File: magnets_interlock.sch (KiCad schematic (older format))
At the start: 18 parts, among them U101 Si8640BD-B-IS

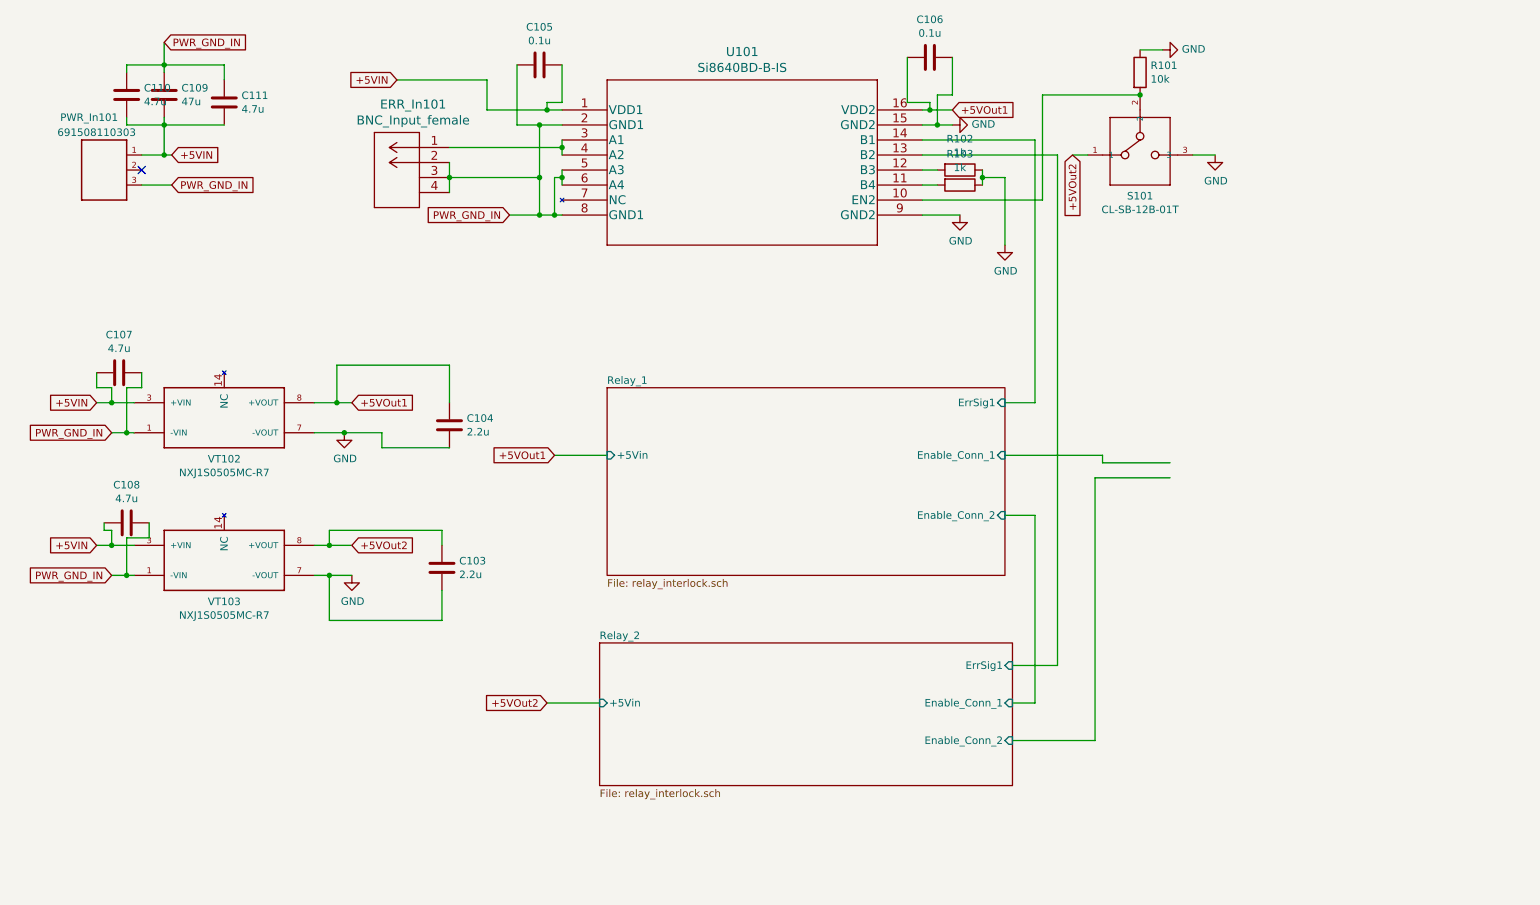
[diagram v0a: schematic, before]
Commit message: Draft 1 Almost There
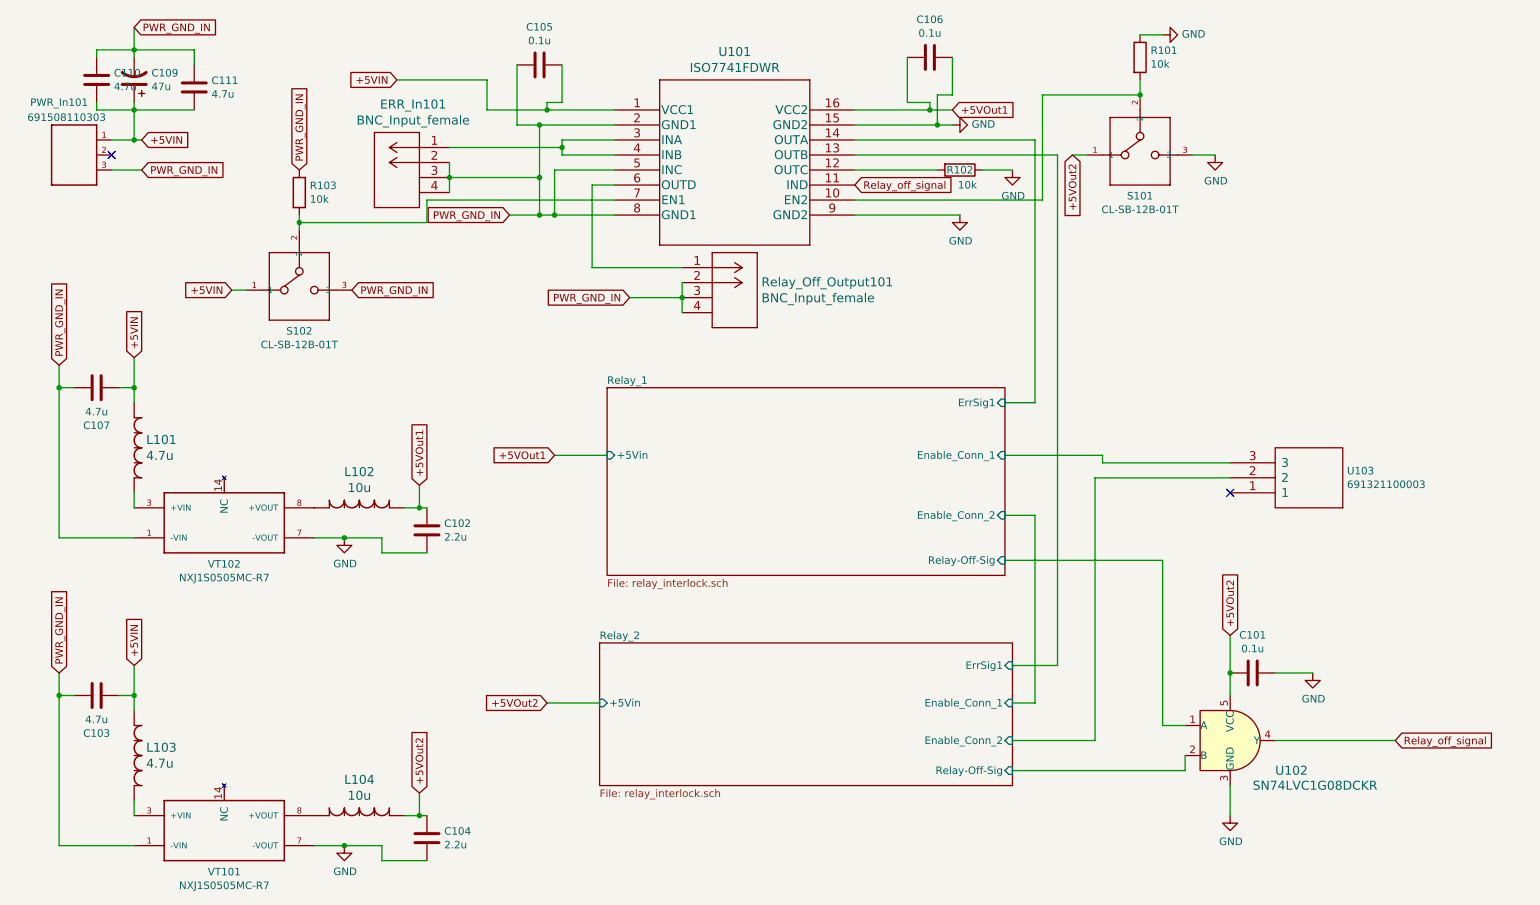
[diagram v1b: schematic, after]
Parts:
- removed C108: 4.7u, Capacitor_SMD:C_1206_3216Metric_Pad1.42x1.75mm_HandSolder, symbol Device:C
- removed C109: 47u, Capacitor_THT:CP_Radial_D8.0mm_P3.50mm, symbol Device:C
- removed U101: Si8640BD-B-IS, SI8640DBIS:Si8640BD-B-IS, symbol 2020-06-26_17-59-50:Si8640BD-B-IS
- removed VT103: NXJ1S0505MC-R7, NXJ1S050:VREG_NXJ1S0505MC-R7, symbol NXJ1S0505MC-R7:NXJ1S0505MC-R7
- added C101: 0.1u, Capacitor_SMD:C_1206_3216Metric_Pad1.42x1.75mm_HandSolder, symbol Device:C
- added C102: 2.2u, Capacitor_SMD:C_1206_3216Metric_Pad1.42x1.75mm_HandSolder, symbol Device:C
- added C109: 47u, Capacitor_THT:CP_Radial_D8.0mm_P3.50mm, symbol Device:CP1
- added L101, L103: 4.7u, VLCF4024T-4R7N1R4-2:VLCF4024T-4R7N1R4-2, symbol 2020-06-30_20-16-32:VLCF4024T-4R7N1R4-2
- added L102, L104: 10u, VLCF4024T-4R7N1R4-2:VLCF4024T-4R7N1R4-2, symbol 2020-06-30_19-50-11:VLCF4024T-100MR90-2
- added Relay_Off_Output101: BNC_Input_female, BNC_female:1-1337543-0, symbol magnets_interlock_library:BNC_Input_female
- added S102: CL-SB-12B-01T, CL-SB-12B-01T:CL-SB-12B, symbol CL-SB-12B-01T:CL-SB-12B-01T
- added U101: ISO7741FDWR, ISO7741FDWR:ISO7741FDWR, symbol 2020-06-30_17-30-58:ISO7741FDWR
- added U102: SN74LVC1G08DCKR, inverter:SN74LVC1G14DCKR, symbol dk_Logic-Gates-and-Inverters:SN74LVC1G08DCKR
- added U103: 691321100003, Magnet_PS_Interlock:691321100003, symbol enrique_3termscrew:691321100003
- added VT101: NXJ1S0505MC-R7, NXJ1S050:VREG_NXJ1S0505MC-R7, symbol NXJ1S0505MC-R7:NXJ1S0505MC-R7
- C103: value 2.2u -> 4.7u
- R102, R103: value 1k -> 10k
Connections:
- net +5VIN: now also C103.1, C109.1, L101.2, L103.2, S102.1, U101.1 (VCC1); no longer VT102.3 (+VIN)
- net +5VOut1: now also C102.1, L102.1, U101.16 (VCC2); no longer C104.1, VT102.8 (+VOUT)
- net +5VOut2: now also C104.1, C101.2, L104.1, U102.5 (VCC); no longer C103.1
- net GND: now also C101.1, C102.2, U101.15 (GND2), U101.9 (GND2), U102.3 (GND), VT101.7 (-VOUT); no longer C103.2, R103.1
- net PWR_GND_IN: now also C103.2, R103.1, C109.2, Relay_Off_Output101.2 (BNC_Shield), Relay_Off_Output101.3 (shield), Relay_Off_Output101.4 (shield), S102.3, U101.2 (GND1), U101.5 (INC), U101.8 (GND1), VT101.1 (-VIN)
- net Relay_1/Enable_Conn_1: now also U103.3
- net Relay_1/ErrSig1: now also U101.14 (OUTA)
- net Relay_2/Enable_Conn_2: now also U103.2
- net Relay_2/ErrSig1: now also U101.13 (OUTB)
- net at R101.2, S101.2: now also U101.10 (EN2)
- net at R103.2: now also S102.2, U101.7 (EN1)
- net at R102.2: now also U101.12 (OUTC)
- net at ERR_In101.1 (Center_Pin): now also U101.3 (INA), U101.4 (INB)
- new net: L101.1, VT102.3 (+VIN)
- new net: L102.2, VT102.8 (+VOUT)
- new net: L104.2, VT101.8 (+VOUT)
- new net: L103.1, VT101.3 (+VIN)
- new net: Relay_Off_Output101.1 (Center_Pin), U101.6 (OUTD)
- new net Relay_1/Relay-Off-Sig: U102.1 (A)
- new net Relay_2/Relay-Off-Sig: U102.2 (B)
- new net Relay_off_signal: U101.11 (IND), U102.4 (Y)
- no-connect marks 1 -> 2
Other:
- moved on the sheet: C107, C110, C111, PWR_In101, R101, VT102

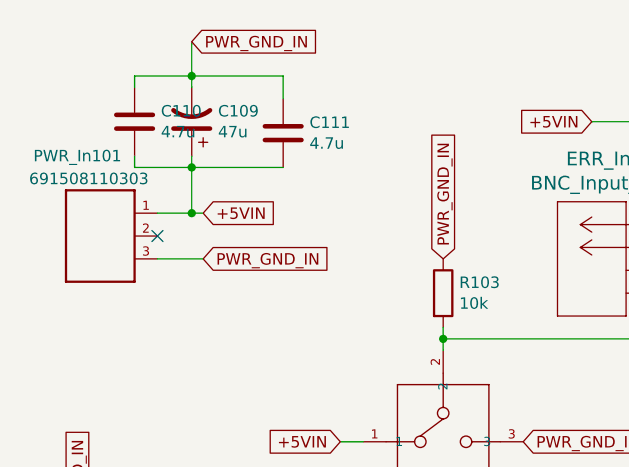
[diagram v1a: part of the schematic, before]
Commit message: Next Draft
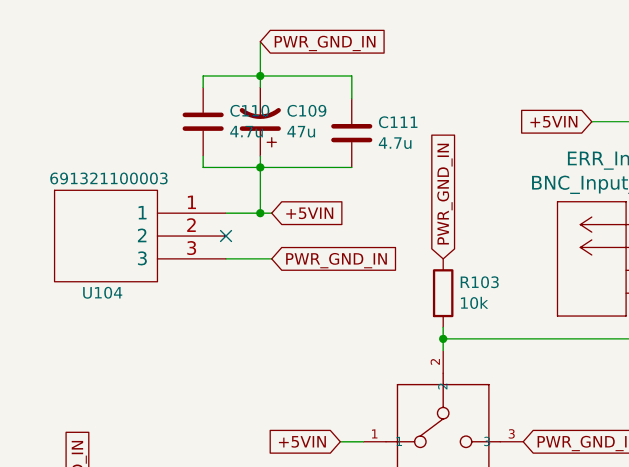
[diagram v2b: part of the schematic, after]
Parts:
- removed PWR_In101: 691508110303, 3PinPowerTerm:691508110303, symbol 691508110303:691508110303
- added U104: 691321100003, Magnet_PS_Interlock:691321100003, symbol enrique_3termscrew:691321100003
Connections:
- net +5VIN: now also U104.1
- net PWR_GND_IN: now also U104.3
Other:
- moved on the sheet: C109, C110, C111
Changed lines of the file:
@@
 Comment4 ""
 $EndDescr
-$Comp
-L 691508110303:691508110303 PWR_In101
-U 1 1 5EF7A439
-P 800 1400
-F 0 "PWR_In101" H 900 1750 50  0000 C CNN
-F 1 "691508110303" H 850 1650 50  0000 C CNN
-F 2 "3PinPowerTerm:691508110303" H 800 1400 50  0001 L BNN
-F 3 "" H 800 1400 50  0001 C CNN
-	1    800  1400
-	-1   0    0    -1
-$EndComp
-Text GLabel 1250 1300 2    50   Input ~ 0
+Text GLabel 1550 1300 2    50   Input ~ 0
 +5VIN
 Wire Wire Line
-	1250 1300 1200 1300
-Text GLabel 1250 1500 2    50   Input ~ 0
+	1550 1300 1500 1300
+Text GLabel 1550 1500 2    50   Input ~ 0
 PWR_GND_IN
 Wire Wire Line
-	1250 1500 1050 1500
-NoConn ~ 1050 1400
+	1550 1500 1350 1500
+NoConn ~ 1350 1400
 $Comp
 L magnets_interlock_library:BNC_Input_female ERR_In101
@@
 	1    0    0    -1
 $EndComp
-Connection ~ 1200 1300
-Wire Wire Line
-	1200 1300 1050 1300
-Text GLabel 1200 550  2    50   Input ~ 0
+Connection ~ 1500 1300
+Wire Wire Line
+	1500 1300 1350 1300
+Text GLabel 1500 550  2    50   Input ~ 0
 PWR_GND_IN
 $Comp
 L Device:C C110
 U 1 1 5F0D1FE9
-P 950 900
-F 0 "C110" H 1065 946 50  0000 L CNN
-F 1 "4.7u" H 1065 855 50  0000 L CNN
-F 2 "Capacitor_SMD:C_1206_3216Metric_Pad1.42x1.75mm_HandSolder" H 988 750 50  0001 C CNN
-F 3 "~" H 950 900 50  0001 C CNN
-	1    950  900
+P 1250 900
+F 0 "C110" H 1365 946 50  0000 L CNN
+F 1 "4.7u" H 1365 855 50  0000 L CNN
+F 2 "Capacitor_SMD:C_1206_3216Metric_Pad1.42x1.75mm_HandSolder" H 1288 750 50  0001 C CNN
+F 3 "~" H 1250 900 50  0001 C CNN
+	1    1250 900
 	1    0    0    -1
 $EndComp
@@
 L Device:C C111
 U 1 1 5F0D256B
-P 1600 950
-F 0 "C111" H 1715 996 50  0000 L CNN
-F 1 "4.7u" H 1715 905 50  0000 L CNN
-F 2 "Capacitor_SMD:C_1206_3216Metric_Pad1.42x1.75mm_HandSolder" H 1638 800 50  0001 C CNN
-F 3 "~" H 1600 950 50  0001 C CNN
-	1    1600 950
-	1    0    0    -1
-$EndComp
-Wire Wire Line
-	1600 1100 1200 1100
-Wire Wire Line
-	1200 1050 1200 1100
-Connection ~ 1200 1100
-Wire Wire Line
-	1200 1100 1200 1300
-Wire Wire Line
-	1200 1100 950  1100
-Wire Wire Line
-	950  1100 950  1050
-Wire Wire Line
-	950  750  950  700
-Wire Wire Line
-	950  700  1200 700
-Connection ~ 1200 700
-Wire Wire Line
-	1200 700  1200 750
-Wire Wire Line
-	1600 800  1600 700
-Wire Wire Line
-	1600 700  1200 700
-Wire Wire Line
-	1200 550  1200 700
+P 1900 950
+F 0 "C111" H 2015 996 50  0000 L CNN
+F 1 "4.7u" H 2015 905 50  0000 L CNN
+F 2 "Capacitor_SMD:C_1206_3216Metric_Pad1.42x1.75mm_HandSolder" H 1938 800 50  0001 C CNN
+F 3 "~" H 1900 950 50  0001 C CNN
+	1    1900 950
+	1    0    0    -1
+$EndComp
+Wire Wire Line
+	1900 1100 1500 1100
+Wire Wire Line
+	1500 1050 1500 1100
+Connection ~ 1500 1100
+Wire Wire Line
+	1500 1100 1500 1300
+Wire Wire Line
+	1500 1100 1250 1100
+Wire Wire Line
+	1250 1100 1250 1050
+Wire Wire Line
+	1250 750  1250 700
+Wire Wire Line
+	1250 700  1500 700
+Connection ~ 1500 700
+Wire Wire Line
+	1500 700  1500 750
+Wire Wire Line
+	1900 800  1900 700
+Wire Wire Line
+	1900 700  1500 700
+Wire Wire Line
+	1500 550  1500 700
 Text GLabel 3700 1800 0    50   Input ~ 0
 PWR_GND_IN
@@
 L Device:CP1 C109
 U 1 1 5EFCC247
-P 1200 900
-F 0 "C109" H 1085 854 50  0000 R CNN
-F 1 "47u" H 1085 945 50  0000 R CNN
-F 2 "Capacitor_THT:CP_Radial_D8.0mm_P3.50mm" H 1200 900 50  0001 C CNN
-F 3 "~" H 1200 900 50  0001 C CNN
-	1    1200 900
+P 1500 900
+F 0 "C109" H 1385 854 50  0000 R CNN
+F 1 "47u" H 1385 945 50  0000 R CNN
+F 2 "Capacitor_THT:CP_Radial_D8.0mm_P3.50mm" H 1500 900 50  0001 C CNN
+F 3 "~" H 1500 900 50  0001 C CNN
+	1    1500 900
 	-1   0    0    1
 $EndComp
@@
 Text GLabel 3100 5650 1    50   Input ~ 0
 +5VOut2
+$Comp
+L enrique_3termscrew:691321100003 U104
+U 1 1 5EFC935A
+P 850 1300
+F 0 "U104" H 900 950 50  0000 R CNN
+F 1 "691321100003" H 1100 1450 50  0000 R CNN
+F 2 "Magnet_PS_Interlock:691321100003" H 850 1300 50  0001 C CNN
+F 3 "" H 850 1300 50  0001 C CNN
+	1    850  1300
+	1    0    0    -1
+$EndComp
 $EndSCHEMATC
